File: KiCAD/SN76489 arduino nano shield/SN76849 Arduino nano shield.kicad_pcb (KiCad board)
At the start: 2 copper layers, 4.4 x 24.3 mm, 1 part, among them U1 PCF8574

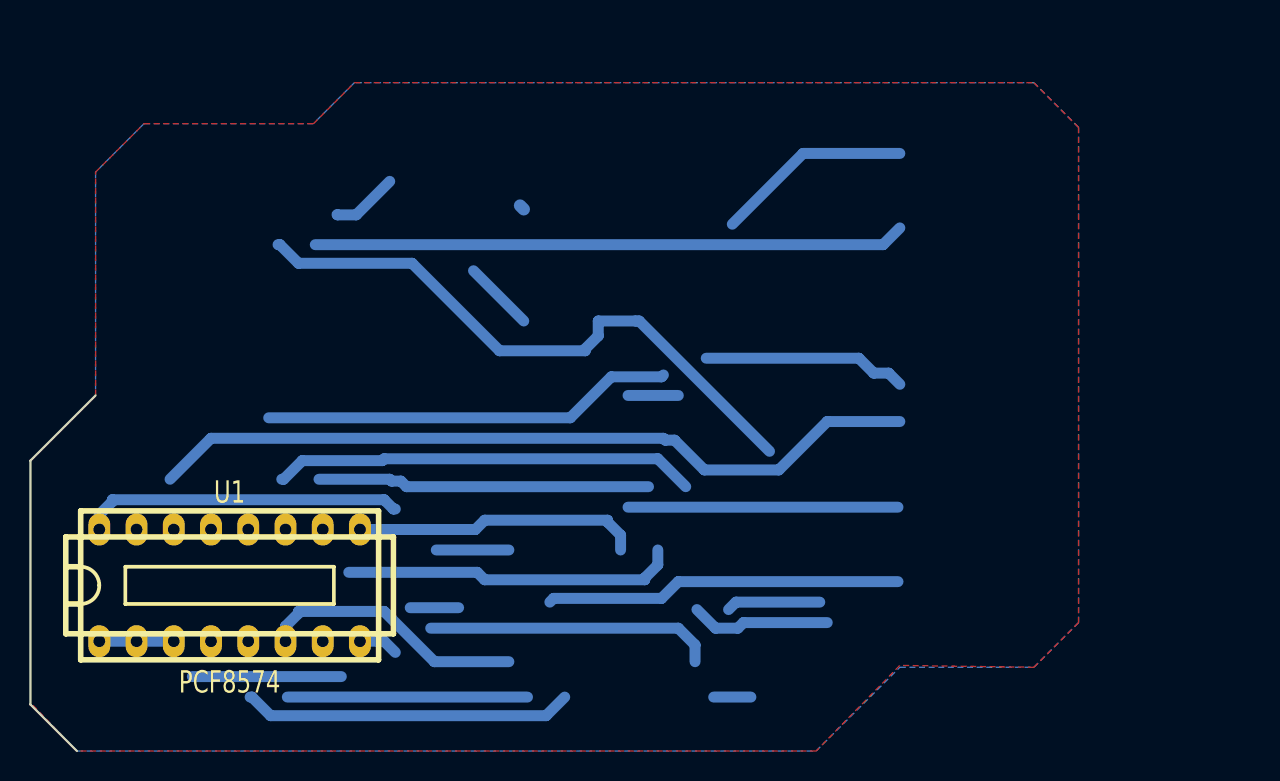
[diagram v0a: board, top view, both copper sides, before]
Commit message: Printplaat 20180601 0.5 laat maak
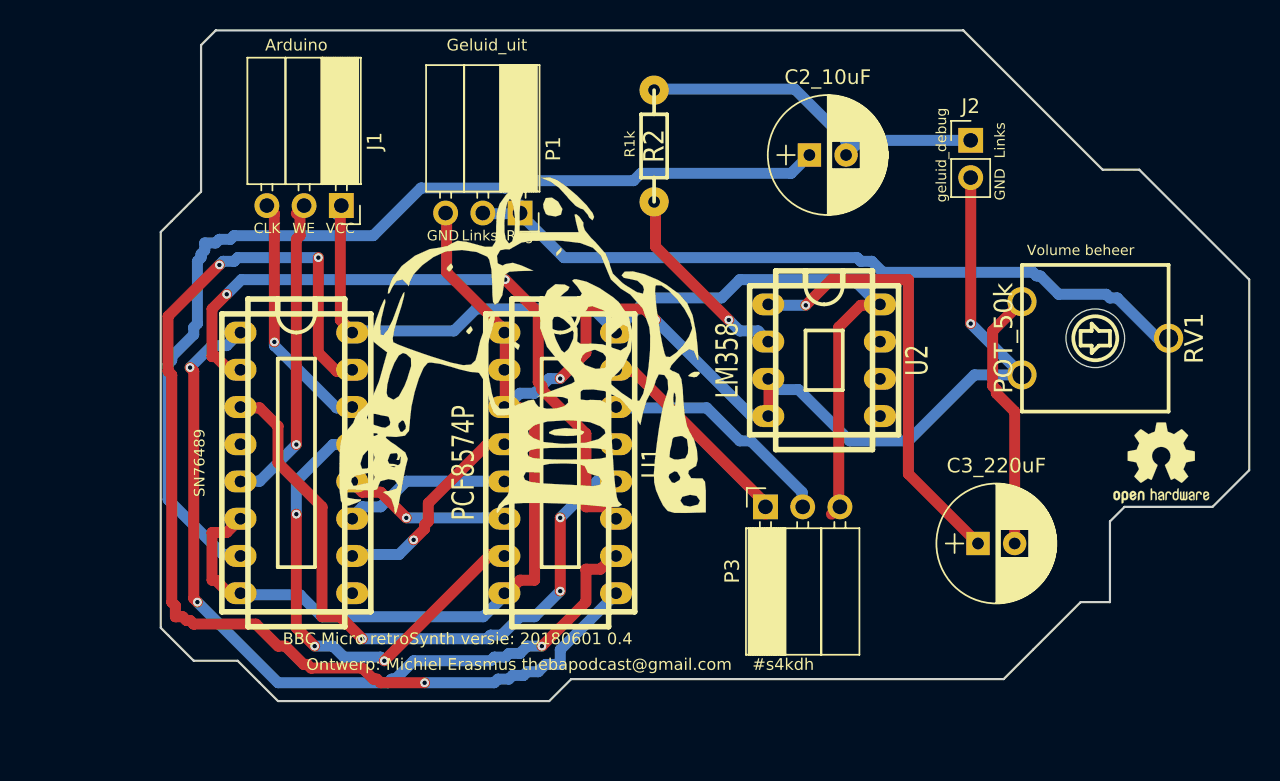
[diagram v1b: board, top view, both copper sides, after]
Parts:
- added C2_10uF: CP_10uF, Capacitors_THT:CP_Radial_D8.0mm_P2.50mm, F.Cu at (68.0, 25.0)
- added C3_220uF: CP_220uF, Capacitors_THT:CP_Radial_D8.0mm_P2.50mm, F.Cu at (79.5, 51.5)
- added G***: LOGO, lib_michiel:Sovjet_simpits_logo01, F.Cu at (48.5, 37.8)
- added J1: Arduino_sn, Socket_Strips:Socket_Strip_Angled_1x03_Pitch2.54mm, F.Cu at (36.1, 28.4)
- added J2: audio_debug, Socket_Strips:Socket_Strip_Straight_1x02_Pitch2.54mm, F.Cu at (79.0, 24.0)
- added P1: Audio_uit, Socket_Strips:Socket_Strip_Angled_1x03_Pitch2.54mm, F.Cu at (48.3, 29.0)
- added P3: I2C, Socket_Strips:Socket_Strip_Angled_1x03_Pitch2.54mm, F.Cu at (65.0, 49.0)
- added R2: R1k, w_pth_resistors:RC03, F.Cu at (57.4, 24.4)
- added REF***: OSHW-Logo, Symbols:OSHW-Logo2_7.3x6mm_SilkScreen, F.Cu at (92.0, 46.0)
- added RV1: POT_50k, w_pth_resistors:trimmer_ecp_ca9-v10, F.Cu at (87.5, 37.5)
- added U2: LM358, w_pth_circuits:dil_8-300_socket, F.Cu at (69.0, 39.0)
- added U3: SN76489, w_pth_circuits:dil_16-300_socket, F.Cu at (33.0, 46.0)
- U1: value PCF8574 -> PCF8574P
- moved U1 24.1 mm to (51.0, 46.0), turned to 270 degrees
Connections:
- net /CE renamed GND
- U1 pad 10: /D2 -> /P5
- U1 pad 11: /D1 -> /P6
- U1 pad 12: /D0 -> /P7
- U1 pad 4: /D7 -> /P0
- U1 pad 5: /D6 -> /P1
- U1 pad 6: /D5 -> /P2
- U1 pad 7: /D4 -> /P3
- U1 pad 9: /D3 -> /P4
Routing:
- net (no net): track 416.6 -> 0.00 mm
- net GND: track 7.81 -> 123.4 mm, vias 0 -> 3
- net /P4: track 0.00 -> 77.1 mm, vias 0 -> 3
- net /Audio: track 0.00 -> 68.9 mm
- net /P5: track 0.00 -> 56.7 mm, vias 0 -> 3
- net Net-(P1-Pad1): track 0.00 -> 52.4 mm
- net /P6: track 0.00 -> 46.8 mm, vias 0 -> 2
- net /P7: track 0.00 -> 45.4 mm, vias 0 -> 3
- net /VCC: track 22.0 -> 65.6 mm
- net /P3: track 0.00 -> 33.2 mm, vias 0 -> 3
- net Net-(C3-Pad1): track 0.00 -> 30.3 mm, vias 0 -> 1
- net Net-(C2-Pad2): track 0.00 -> 24.6 mm
- net /WE: track 0.00 -> 22.1 mm, vias 0 -> 1
- net /D3: track 19.6 -> 0.00 mm
- net /D5: track 18.2 -> 0.00 mm
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- removed copper zone on B.Cu, net (none)
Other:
- board size 4.4 x 24.3 mm -> 74.2 x 45.8 mm
- board text added: "Arduino"
- board text added: "BBC Micro retroSynth versie: 20180601 0.4"
- board text added: "CLK"
- board text added: "Elkeen het ingebore waardigheid en die reg dat daardie waardigheid gerespekteer en beskerm word."
- board text added: "GND"
- board text added: "Geluid_uit"
- board text added: "Links"
- board text added: "Ontwerp: Michiel Erasmus thebapodcast@gmail.com #s4kdh"
- board text added: "R1k"
- board text added: "Regs"
- board text added: "VCC"
- board text added: "Volume beheer"
- board text added: "WE"
- board text added: "geluid_debug"
